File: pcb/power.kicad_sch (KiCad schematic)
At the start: 20 parts, among them J5 PWR IN, J6 Raspberry_Pi_4, Q1 AO3401A, U5 TPS5430DDA

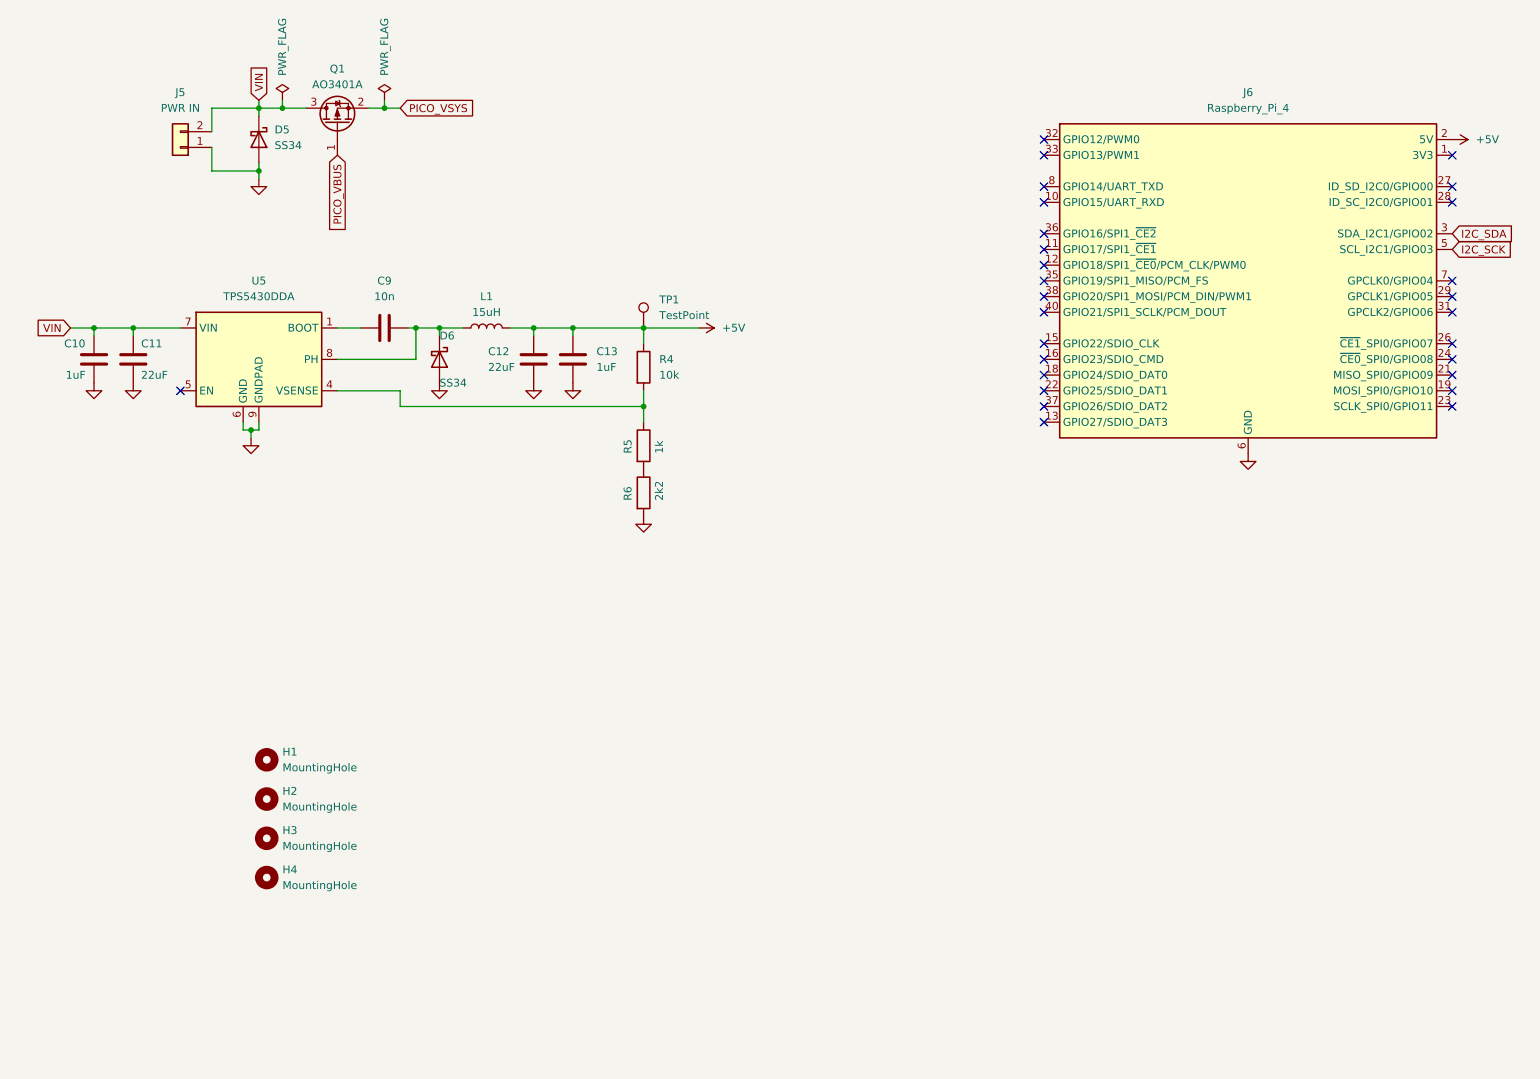
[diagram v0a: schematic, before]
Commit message: wip on the pcb
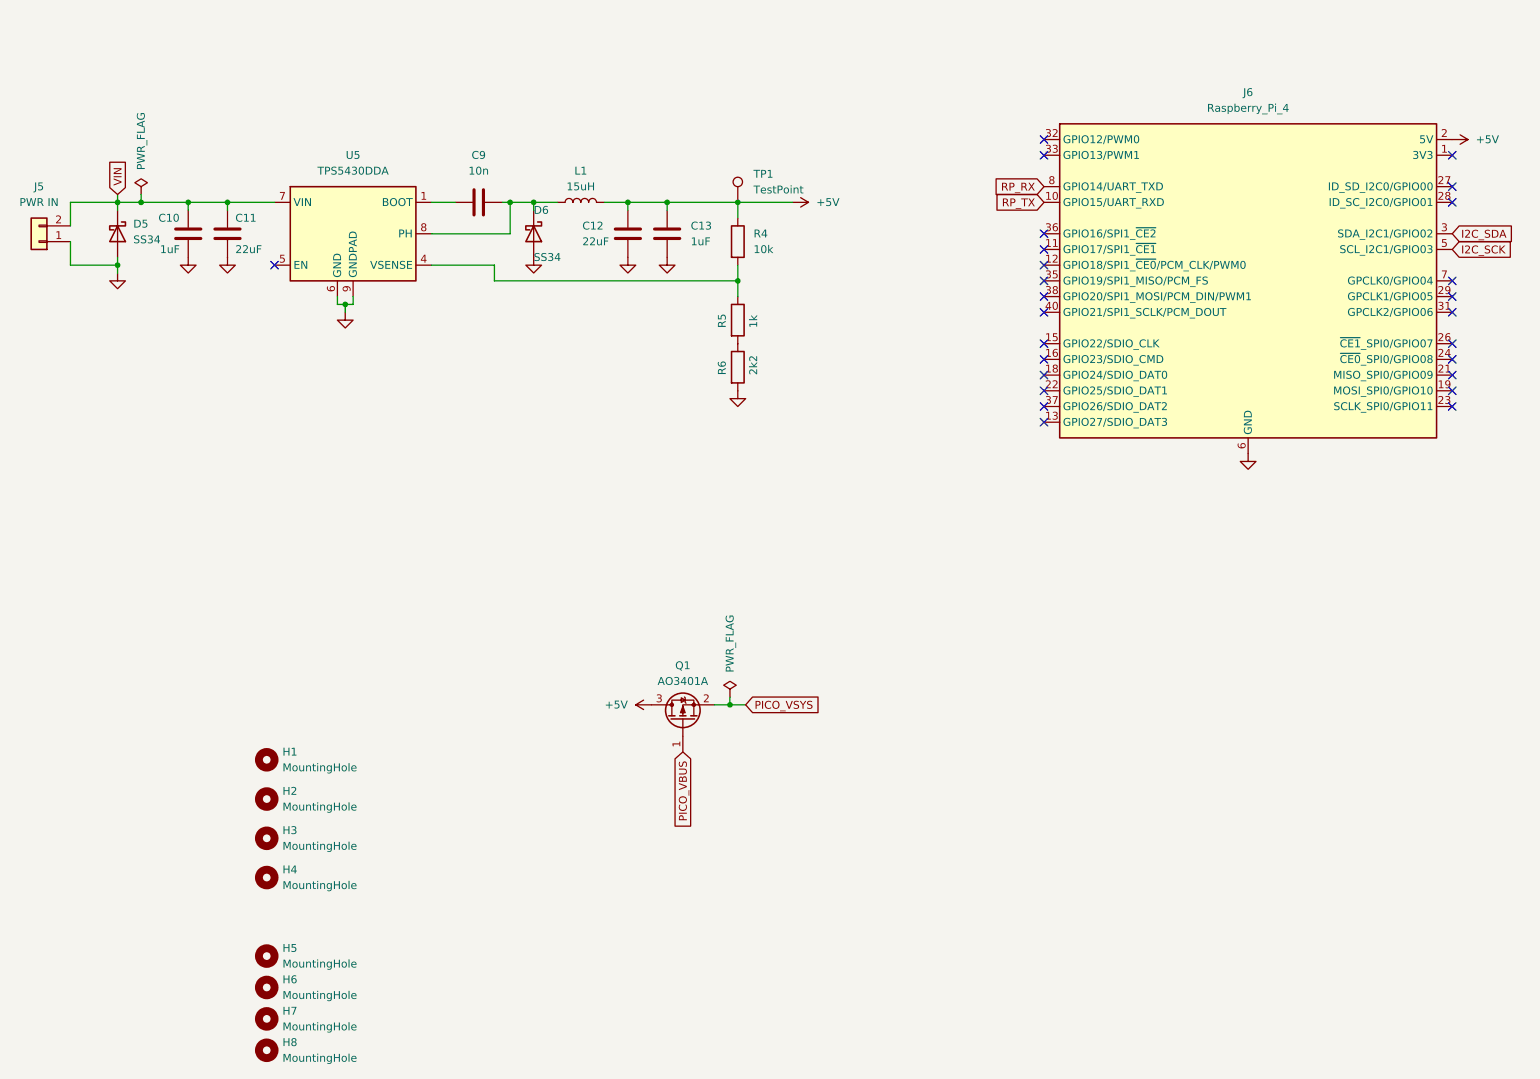
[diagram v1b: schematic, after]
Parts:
- added H5, H6, H7, H8: MountingHole, MountingHole:MountingHole_2.2mm_M2, symbol Mechanical:MountingHole
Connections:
- net +5V: now also Q1.3 (D)
- net VIN: no longer Q1.3 (D)
- net RP_TX: now reaches J6.10 (GPIO15/UART_RXD)
- net RP_RX: now reaches J6.8 (GPIO14/UART_TXD)
- no-connect marks 28 -> 26
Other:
- moved on the sheet: C10, C11, C12, C13, C9, D5, D6, J5, L1, Q1, R4, R5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
